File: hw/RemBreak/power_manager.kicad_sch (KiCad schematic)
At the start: 20 parts, among them IC1 LTC2943IDD#TRPBF, J10 Screw_Terminal_01x02, J11 Conn_01x03, Q4 BC337, Q5 BC847, U6 INA219BxDCN, U7 MAX40200AUK

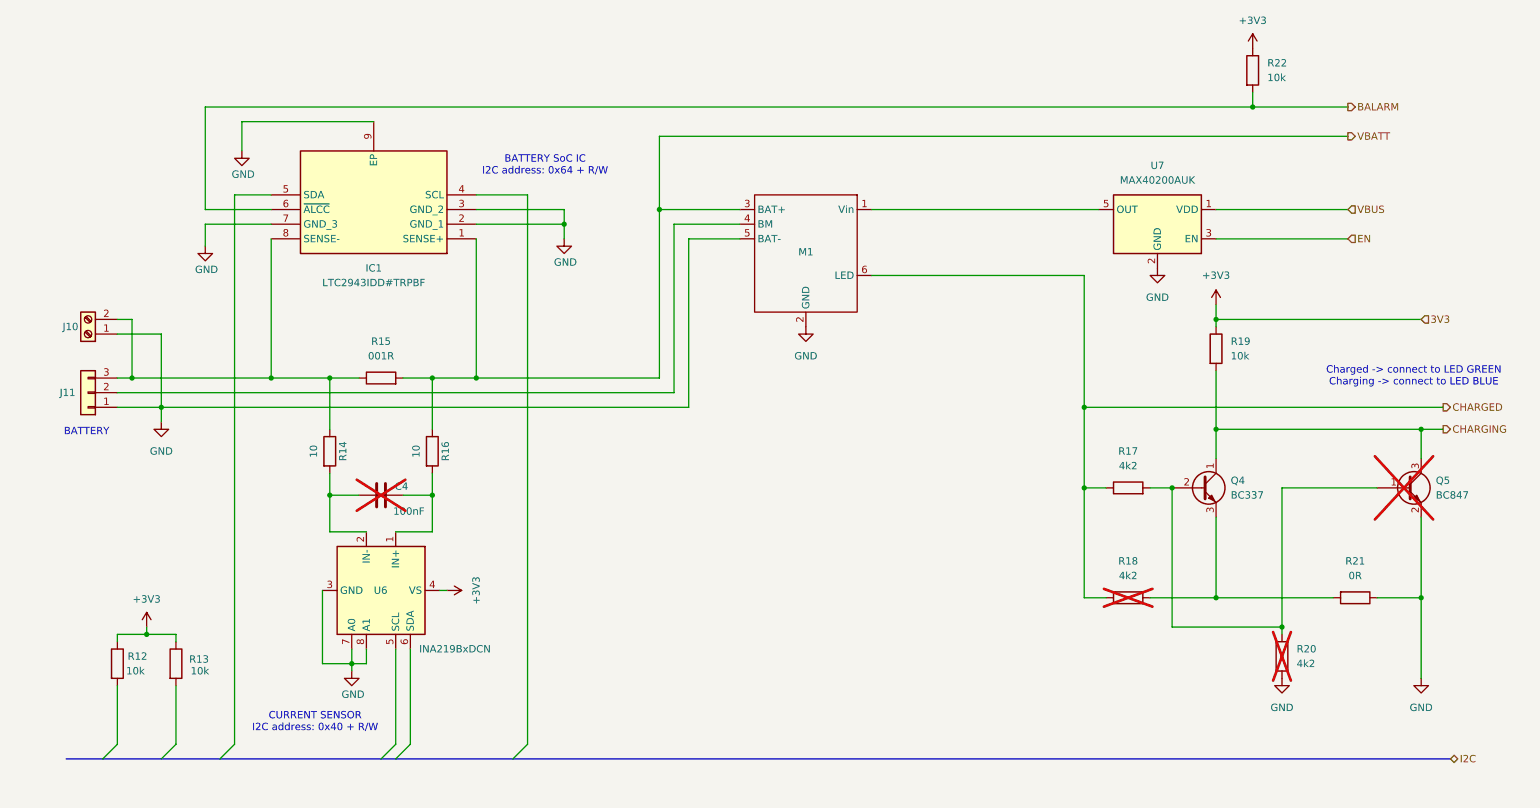
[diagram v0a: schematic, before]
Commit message: finished schematics routing and erc passed
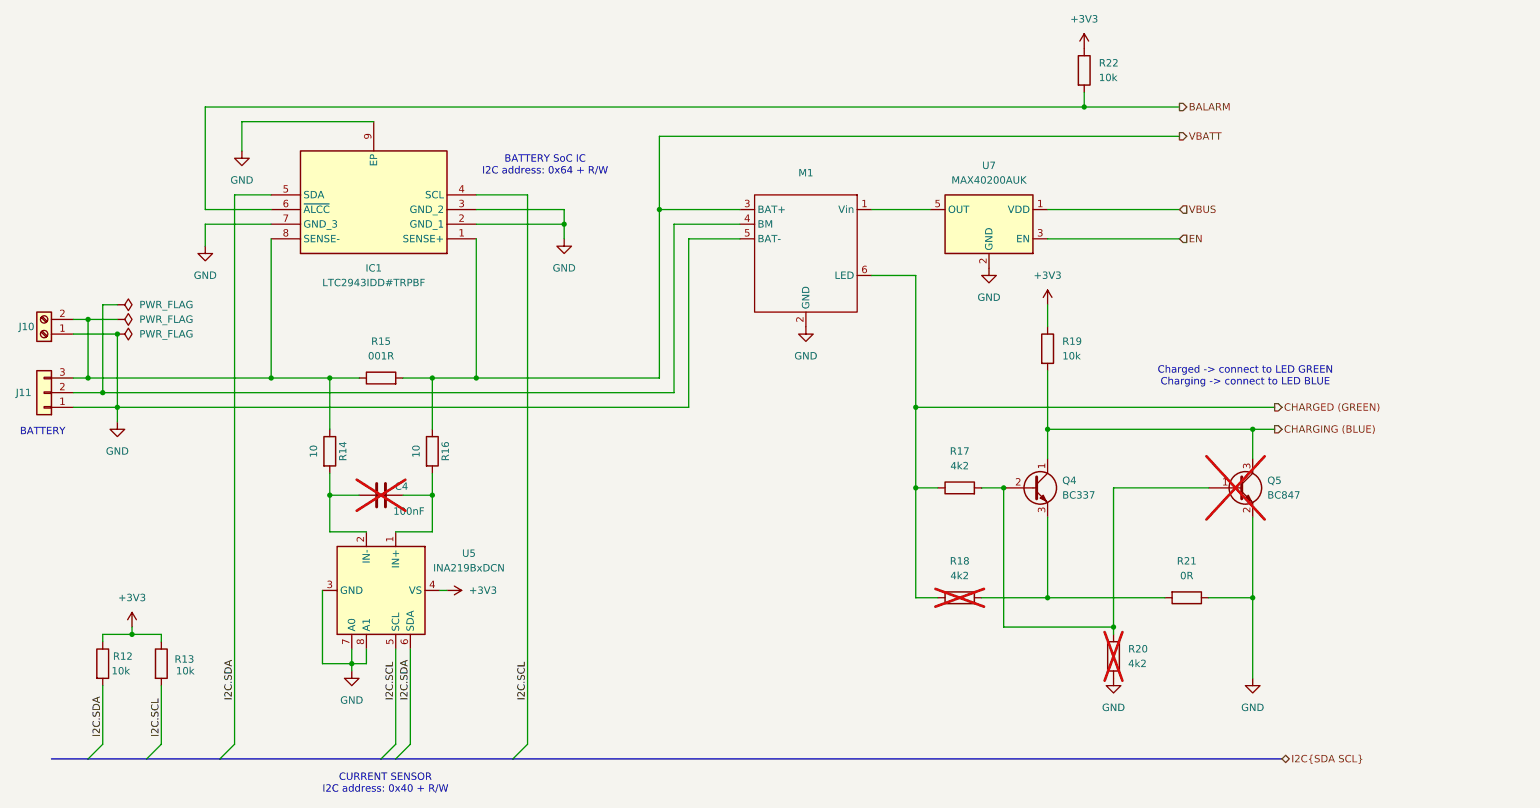
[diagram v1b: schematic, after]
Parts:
- removed U6: INA219BxDCN, Package_TO_SOT_SMD:SOT-23-8, symbol Analog_ADC:INA219BxDCN
- added U5: INA219BxDCN, Package_TO_SOT_SMD:SOT-23-8, symbol Sensor_Energy:INA219BxDCN
- IC1: footprint Package_DFN_QFN:DFN-8-1EP_3x3mm_P0.5mm_EP1.7x2.4mm -> Package_DFN_QFN:DFN-8-1EP_3x3mm_P0.5mm_EP1.66x2.38mm
- M1: footprint chinese_modules:USBC_charger -> (none)
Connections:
- net +3V3: now also U5.4 (VS)
- net GND: now also U5.3 (GND), U5.7 (A0), U5.8 (A1)
- net I2C.SCL: now reaches R13.2
- net I2C.SCL: now also IC1.4 (SCL), U5.5 (SCL)
- net I2C.SDA: now reaches IC1.5 (SDA)
- net I2C.SDA: now also R12.2, U5.6 (SDA)
- net at C4.1, R14.2: now also U5.2 (IN-)
- net at C4.2, R16.2: now also U5.1 (IN+)
- net CHARGED renamed CHARGED (GREEN)
- net CHARGING renamed CHARGING (BLUE)
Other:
- moved on the sheet: J10, J11, Q4, Q5, R12, R13, R17, R18, R19, R20, R21, R22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
